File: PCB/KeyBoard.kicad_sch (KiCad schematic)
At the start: 196 parts, among them P1 USB_C_Plug_USB2.0, P2 USB_C_Plug_USB2.0, SW1 SW_Push, SW10 SW_Push, SW11 SW_Push, SW12 SW_Push, SW13 SW_Push, SW14 SW_Push, SW15 SW_Push, SW16 SW_Push, SW17 SW_Push, SW18 SW_Push, SW19 SW_Push, SW2 SW_Push, SW20 SW_Push, SW21 SW_Push, SW22 SW_Push, SW23 SW_Push, SW24 SW_Push, SW25 SW_Push, SW26 SW_Push, SW27 SW_Push, SW28 SW_Push, SW29 SW_Push, SW3 SW_Push, SW30 SW_Push, SW31 SW_Push, SW32 SW_Push, SW33 SW_Push, SW34 SW_Push, SW35 SW_Push, SW36 SW_Push, SW37 SW_Push, SW38 SW_Push, SW39 SW_Push, SW4 SW_Push, SW40 SW_Push, SW41 SW_Push, SW42 SW_Push, SW43 SW_Push, SW44 SW_Push, SW45 SW_Push, SW46 SW_Push, SW47 SW_Push, SW48 SW_Push, SW49 SW_Push, SW5 SW_Push, SW50 SW_Push, SW51 SW_Push, SW52 SW_Push, SW53 SW_Push, SW54 SW_Push, SW55 SW_Push, SW56 SW_Push, SW57 SW_Push, SW58 SW_Push, SW59 SW_Push, SW6 SW_Push, SW60 SW_Push, SW61 SW_Push, SW64 RotaryEncoder_Switch_MP, SW7 SW_Push, SW8 SW_Push, SW9 SW_Push, U1 PCA9555D, U2 PCA9555D, U3 XIAO-RP2040-DIP

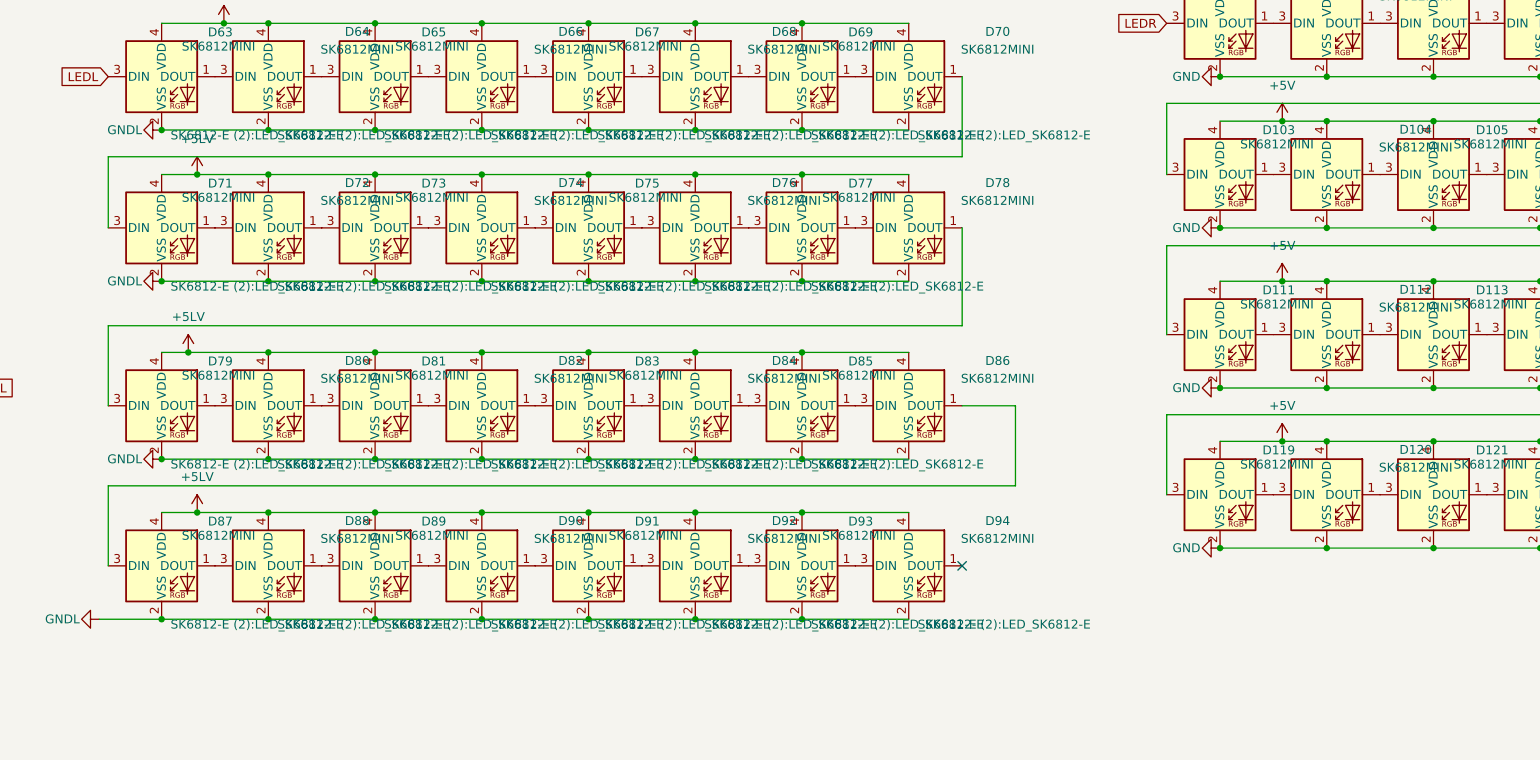
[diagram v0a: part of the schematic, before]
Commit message: Add files via upload
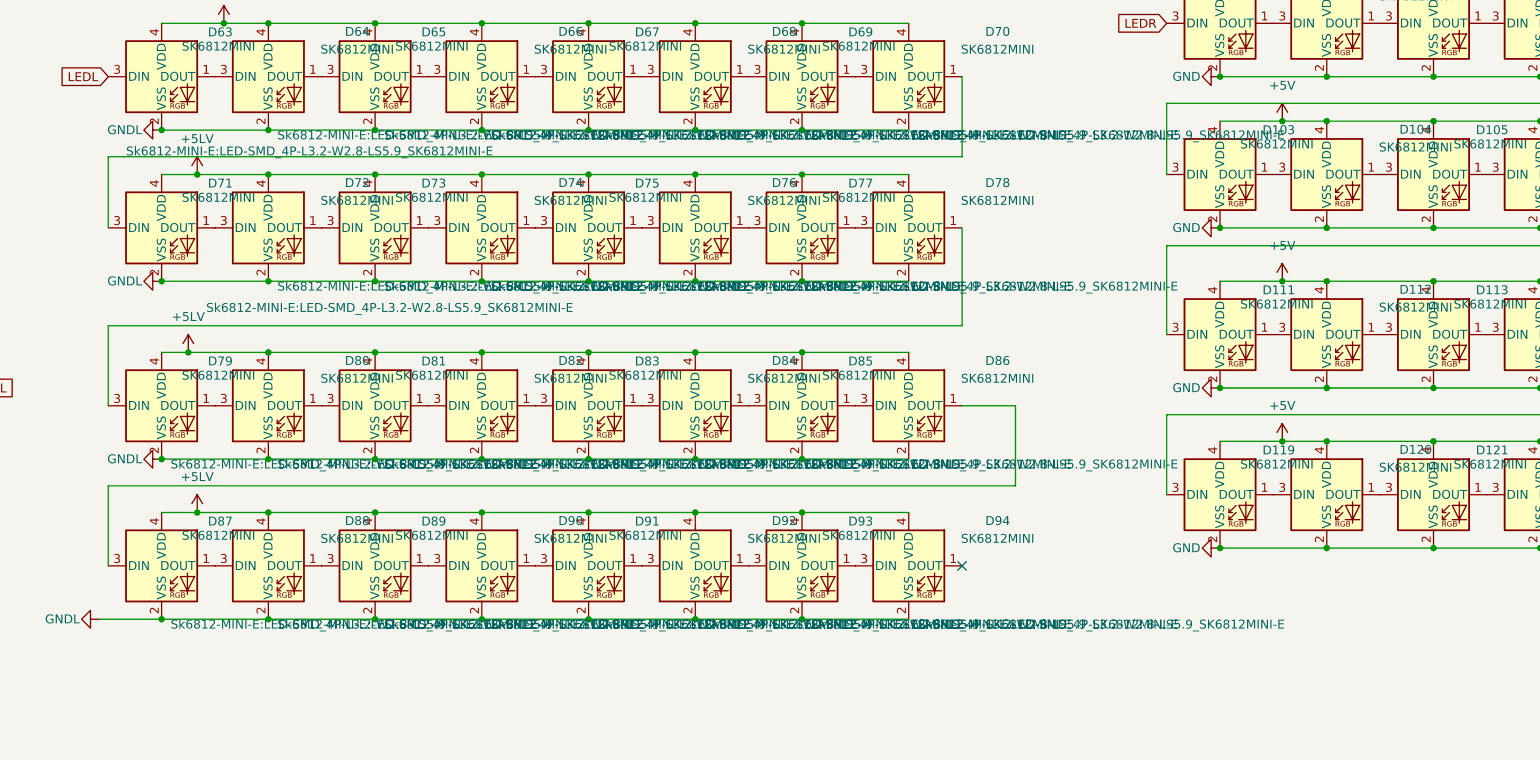
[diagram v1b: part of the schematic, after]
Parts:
- D100, D101, D102, D103, D104, D105, D106, D107, D108, D109, D110, D111, D112, D113, D114, D115, D116, D117, D118, D119, D120, D121, D122, D123, D63, D64, D65, D66, D67, D68, D69, D70, D71, D72, D73, D74, D75, D76, D77, D78, D79, D80, D81, D82, D83, D84, D85, D86, D87, D88, D89, D90, D91, D92, D93, D94, D95, D96, D97, D98, D99: footprint SK6812-E (2):LED_SK6812-E -> Sk6812-MINI-E:LED-SMD_4P-L3.2-W2.8-LS5.9_SK6812MINI-E

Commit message: Add files via upload
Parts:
- removed D100, D101, D102, D103, D104, D105, D106, D107, D108, D109, D110, D111, D112, D113, D114, D115, D116, D117, D118, D119, D120, D121, D122, D123, D63, D64, D65, D66, D67, D68, D69, D70, D71, D72, D73, D74, D75, D76, D77, D78, D79, D80, D81, D82, D83, D84, D85, D86, D87, D88, D89, D90, D91, D92, D93, D94, D95, D96, D97, D98, D99: SK6812MINI, Sk6812-MINI-E:LED-SMD_4P-L3.2-W2.8-LS5.9_SK6812MINI-E, symbol LED:SK6812MINI
- added LED1, LED10, LED11, LED12, LED13, LED14, LED15, LED16, LED17, LED18, LED19, LED2, LED20, LED21, LED22, LED23, LED24, LED25, LED26, LED27, LED28, LED29, LED3, LED30, LED31, LED32, LED33, LED34, LED35, LED36, LED37, LED38, LED39, LED4, LED40, LED41, LED42, LED43, LED44, LED45, LED46, LED47, LED48, LED49, LED5, LED50, LED51, LED52, LED53, LED54, LED55, LED57, LED58, LED59, LED6, LED61, LED62, LED63, LED7, LED8, LED9: SK6812MINI-E_C5149201, Sk6812-MINI-E:LED-SMD_4P-L3.2-W2.8-LS5.9_SK6812MINI-E, symbol kikiki:SK6812MINI-E_C5149201
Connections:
- net +5LV: now also LED1.3 (VDD), LED10.3 (VDD), LED11.3 (VDD), LED12.3 (VDD), LED13.3 (VDD), LED14.3 (VDD), LED15.3 (VDD), LED16.3 (VDD), LED17.3 (VDD), LED18.3 (VDD), LED19.3 (VDD), LED2.3 (VDD), LED20.3 (VDD), LED21.3 (VDD), LED22.3 (VDD), LED23.3 (VDD), LED24.3 (VDD), LED25.3 (VDD), LED26.3 (VDD), LED27.3 (VDD), LED28.3 (VDD), LED29.3 (VDD), LED3.3 (VDD), LED30.3 (VDD), LED31.3 (VDD), LED32.3 (VDD), LED4.3 (VDD), LED5.3 (VDD), LED6.3 (VDD), LED7.3 (VDD), LED8.3 (VDD), LED9.3 (VDD)
- net +5V: now also LED33.3 (VDD), LED34.3 (VDD), LED35.3 (VDD), LED36.3 (VDD), LED37.3 (VDD), LED38.3 (VDD), LED39.3 (VDD), LED40.3 (VDD), LED41.3 (VDD), LED42.3 (VDD), LED43.3 (VDD), LED44.3 (VDD), LED45.3 (VDD), LED46.3 (VDD), LED47.3 (VDD), LED48.3 (VDD), LED49.3 (VDD), LED50.3 (VDD), LED51.3 (VDD), LED52.3 (VDD), LED53.3 (VDD), LED54.3 (VDD), LED55.3 (VDD), LED57.3 (VDD), LED58.3 (VDD), LED59.3 (VDD), LED61.3 (VDD), LED62.3 (VDD), LED63.3 (VDD)
- net GND: now also LED33.1 (GND), LED34.1 (GND), LED35.1 (GND), LED36.1 (GND), LED37.1 (GND), LED38.1 (GND), LED39.1 (GND), LED40.1 (GND), LED41.1 (GND), LED42.1 (GND), LED43.1 (GND), LED44.1 (GND), LED45.1 (GND), LED46.1 (GND), LED47.1 (GND), LED48.1 (GND), LED49.1 (GND), LED50.1 (GND), LED51.1 (GND), LED52.1 (GND), LED53.1 (GND), LED54.1 (GND), LED55.1 (GND), LED57.1 (GND), LED58.1 (GND), LED59.1 (GND), LED61.1 (GND), LED62.1 (GND), LED63.1 (GND)
- net GNDL: now also LED1.1 (GND), LED10.1 (GND), LED11.1 (GND), LED12.1 (GND), LED13.1 (GND), LED14.1 (GND), LED15.1 (GND), LED16.1 (GND), LED17.1 (GND), LED18.1 (GND), LED19.1 (GND), LED2.1 (GND), LED20.1 (GND), LED21.1 (GND), LED22.1 (GND), LED23.1 (GND), LED24.1 (GND), LED25.1 (GND), LED26.1 (GND), LED27.1 (GND), LED28.1 (GND), LED29.1 (GND), LED3.1 (GND), LED30.1 (GND), LED31.1 (GND), LED32.1 (GND), LED4.1 (GND), LED5.1 (GND), LED6.1 (GND), LED7.1 (GND), LED8.1 (GND), LED9.1 (GND)
- net LEDL: now also LED1.2 (DIN)
- net LEDR: now also LED33.2 (DIN)
- new net: LED47.4 (DOUT), LED48.2 (DIN)
- new net: LED48.4 (DOUT), LED49.2 (DIN)
- new net: LED23.4 (DOUT), LED24.2 (DIN)
- new net: LED24.4 (DOUT), LED25.2 (DIN)
- new net: LED36.4 (DOUT), LED37.2 (DIN)
- new net: LED37.4 (DOUT), LED38.2 (DIN)
- new net: LED27.4 (DOUT), LED28.2 (DIN)
- new net: LED28.4 (DOUT), LED29.2 (DIN)
- new net: LED54.4 (DOUT), LED55.2 (DIN)
- new net: LED55.4 (DOUT), LED57.2 (DIN)
- new net: LED2.4 (DOUT), LED3.2 (DIN)
- new net: LED3.4 (DOUT), LED4.2 (DIN)
- new net: LED25.4 (DOUT), LED26.2 (DIN)
- new net: LED26.4 (DOUT), LED27.2 (DIN)
- new net: LED35.4 (DOUT), LED36.2 (DIN)
- new net: LED22.4 (DOUT), LED23.2 (DIN)
- new net: LED16.4 (DOUT), LED17.2 (DIN)
- new net: LED17.4 (DOUT), LED18.2 (DIN)
- new net: LED39.4 (DOUT), LED40.2 (DIN)
- new net: LED40.4 (DOUT), LED41.2 (DIN)
- new net: LED50.4 (DOUT), LED51.2 (DIN)
- new net: LED51.4 (DOUT), LED52.2 (DIN)
- new net: LED4.4 (DOUT), LED5.2 (DIN)
- new net: LED5.4 (DOUT), LED6.2 (DIN)
- new net: LED49.4 (DOUT), LED50.2 (DIN)
- new net: LED29.4 (DOUT), LED30.2 (DIN)
- new net: LED6.4 (DOUT), LED7.2 (DIN)
- new net: LED7.4 (DOUT), LED8.2 (DIN)
- new net: LED21.4 (DOUT), LED22.2 (DIN)
- new net: LED38.4 (DOUT), LED39.2 (DIN)
- new net: LED1.4 (DOUT), LED2.2 (DIN)
- new net: LED57.4 (DOUT), LED58.2 (DIN)
- new net: LED59.4 (DOUT), LED61.2 (DIN)
- new net: LED61.4 (DOUT), LED62.2 (DIN)
- new net: LED44.4 (DOUT), LED45.2 (DIN)
- new net: LED45.4 (DOUT), LED46.2 (DIN)
- new net: LED8.4 (DOUT), LED9.2 (DIN)
- new net: LED10.2 (DIN), LED9.4 (DOUT)
- new net: LED19.4 (DOUT), LED20.2 (DIN)
- new net: LED20.4 (DOUT), LED21.2 (DIN)
- new net: LED33.4 (DOUT), LED34.2 (DIN)
- new net: LED34.4 (DOUT), LED35.2 (DIN)
- new net: LED12.4 (DOUT), LED13.2 (DIN)
- new net: LED13.4 (DOUT), LED14.2 (DIN)
- new net: LED11.4 (DOUT), LED12.2 (DIN)
- new net: LED46.4 (DOUT), LED47.2 (DIN)
- new net: LED30.4 (DOUT), LED31.2 (DIN)
- new net: LED31.4 (DOUT), LED32.2 (DIN)
- new net: LED41.4 (DOUT), LED42.2 (DIN)
- new net: LED52.4 (DOUT), LED53.2 (DIN)
- new net: LED18.4 (DOUT), LED19.2 (DIN)
- new net: LED53.4 (DOUT), LED54.2 (DIN)
- new net: LED10.4 (DOUT), LED11.2 (DIN)
- new net: LED42.4 (DOUT), LED43.2 (DIN)
- new net: LED43.4 (DOUT), LED44.2 (DIN)
- new net: LED62.4 (DOUT), LED63.2 (DIN)
- new net: LED15.4 (DOUT), LED16.2 (DIN)
- new net: LED58.4 (DOUT), LED59.2 (DIN)
- new net: LED14.4 (DOUT), LED15.2 (DIN)
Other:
- moved on the sheet: D1, D10, D11, D12, D13, D14, D15, D16, D17, D18, D19, D2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
